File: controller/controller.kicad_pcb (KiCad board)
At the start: 4 copper layers, 30 x 60 mm, 74 parts, among them SW1 SW_SPDT, SW2 SW_SPST

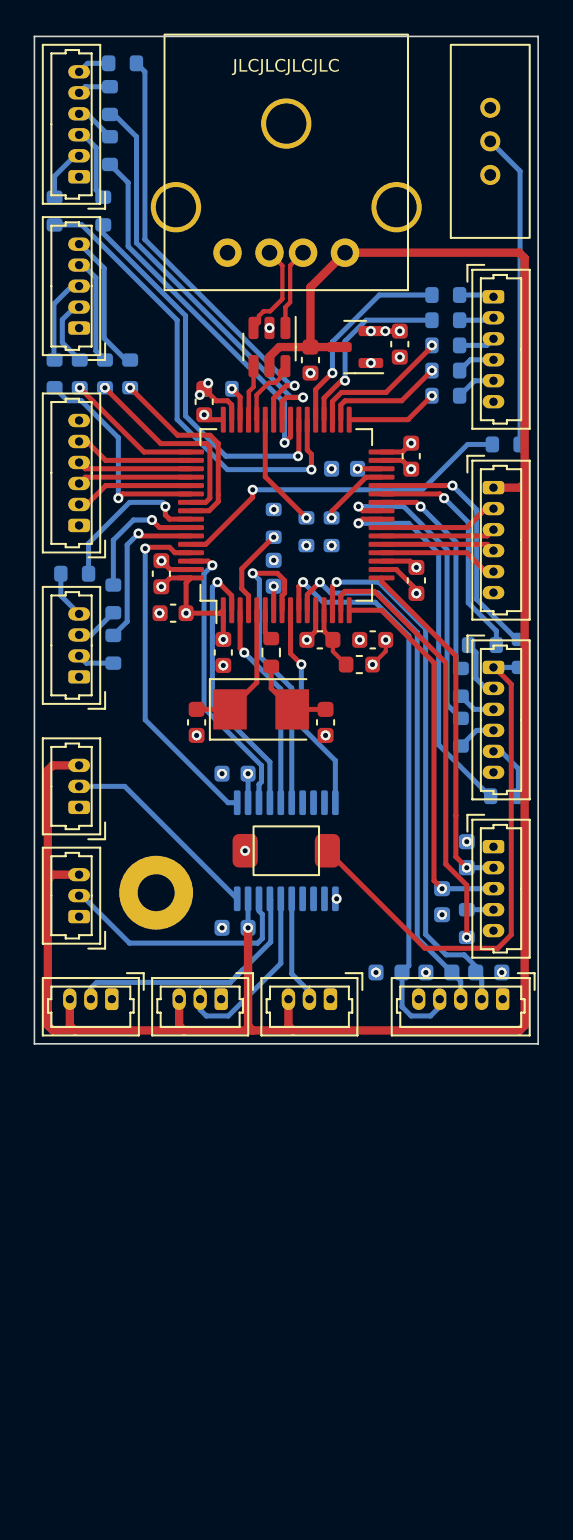
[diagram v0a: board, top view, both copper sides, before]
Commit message: update controller and host boards
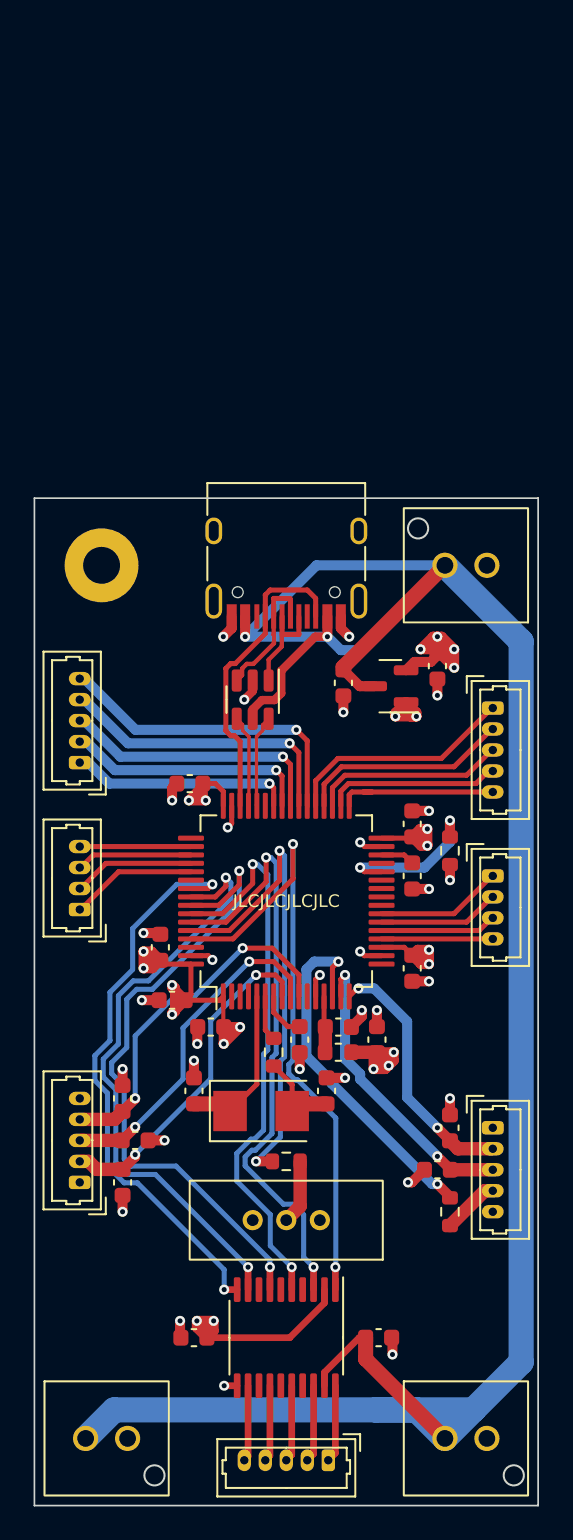
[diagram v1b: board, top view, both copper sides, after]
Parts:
- removed ESD1: USBLC6-2SC6, Package_TO_SOT_SMD:SOT-23-6
- removed H10, H11, H12, H13, H14: Conn_01x03, Connector_Molex:Molex_PicoBlade_53047-0310_1x03_P1.25mm_Vertical
- removed H2, H4, H5, H6: Conn_01x06, Connector_Molex:Molex_PicoBlade_53047-0610_1x06_P1.25mm_Vertical
- removed H3, H8, H9: Conn_01x05, Connector_Molex:Molex_PicoBlade_53047-0510_1x05_P1.25mm_Vertical
- removed H7: Conn_01x04, Connector_Molex:Molex_PicoBlade_53047-0410_1x04_P1.25mm_Vertical
- removed LDO1: AP2127N-3.3, Package_TO_SOT_SMD:SOT-23
- removed MCU1: STM32F401RCT6, Package_QFP:LQFP-64_10x10mm_P0.5mm
- removed MNT1: MountingHole, MountingHole:MountingHole_2.2mm_M2_Pad
- removed R10, R11, R12, R13, R14, R15, R16, R17, R18, R19, R20, R21, R22, R23, R24, R25, R26, R27, R28, R29, R5, R6, R7, R8, R9: 10KR, Resistor_SMD:R_0603_1608Metric
- removed SW2: SW_SPST, Custom:ALPS_SKRKAEE020
- removed USB1: USB_A, Custom:JST_UBA-4R-D14T-4D
- removed VT1: TXS0108EPW, Package_SO:TSSOP-20_4.4x6.5mm_P0.65mm
- removed XTAL1: 8MHz, Crystal:Crystal_SMD_5032-2Pin_5.0x3.2mm
- added J1: Conn_01x02, klib:MOLEX_533750210-Mini-Lock-2Pin-Through-Hole, F.Cu at (135.7, 74.0)
- added J10: Conn_01x05, Connector_Molex:Molex_PicoBlade_53047-0510_1x05_P1.25mm_Vertical, F.Cu at (137.3, 107.5)
- added J11: Conn_01x02, klib:MOLEX_533750210-Mini-Lock-2Pin-Through-Hole, F.Cu at (135.7, 126.0)
- added J2: USB_C_Receptacle_USB2.0, Connector_USB:USB_C_Receptacle_HRO_TYPE-C-31-M-12, F.Cu at (125.0, 73.0)
- added J3: Conn_01x02, klib:MOLEX_533750210-Mini-Lock-2Pin-Through-Hole, F.Cu at (114.3, 126.0)
- added J4: Conn_01x05, Connector_Molex:Molex_PicoBlade_53047-0510_1x05_P1.25mm_Vertical, F.Cu at (127.5, 127.3)
- added J5: Conn_01x04, Connector_Molex:Molex_PicoBlade_53047-0410_1x04_P1.25mm_Vertical, F.Cu at (112.7, 94.5)
- added J6: Conn_01x04, Connector_Molex:Molex_PicoBlade_53047-0410_1x04_P1.25mm_Vertical, F.Cu at (137.3, 92.5)
- added J7: Conn_01x05, Connector_Molex:Molex_PicoBlade_53047-0510_1x05_P1.25mm_Vertical, F.Cu at (112.7, 85.8)
- added J8: Conn_01x05, Connector_Molex:Molex_PicoBlade_53047-0510_1x05_P1.25mm_Vertical, F.Cu at (137.3, 82.5)
- added J9: Conn_01x05, Connector_Molex:Molex_PicoBlade_53047-0510_1x05_P1.25mm_Vertical, F.Cu at (112.7, 110.8)
- added U1: AP2127N-3.3, Package_TO_SOT_SMD:SOT-23, F.Cu at (131.2, 81.2)
- added U2: STM32F401RCT6, Package_QFP:LQFP-64_10x10mm_P0.5mm, F.Cu at (125.0, 94.0)
- added U3: USBLC6-2SC6, Package_TO_SOT_SMD:SOT-23-6, F.Cu at (123.0, 82.0)
- added U4: TXS0108EPW, Package_SO:TSSOP-20_4.4x6.5mm_P0.65mm, F.Cu at (125.0, 120.0)
- added Y1: 8M, Crystal:Crystal_SMD_5032-2Pin_5.0x3.2mm, F.Cu at (123.5, 106.5)
- C1, C2, C3, C9: value 10uF -> 10u
- C10, C4, C5, C6, C7, C8: value 100nF -> 100n
- C11: value 4.7uF -> 20p; moved to F.Cu
- C12: value 100nF -> 20p; moved to F.Cu
- C13: value 20pF -> 4.7u
- C14: value 20pF -> 100n
- C15, C16, C17, C18, C19, C20, C21: value 100nF -> 100n; moved to F.Cu
- H1: value Conn_01x06 -> MountingHole; footprint Connector_Molex:Molex_PicoBlade_53047-0610_1x06_P1.25mm_Vertical -> MountingHole:MountingHole_2.2mm_M2_Pad
- R1: value 0R -> 0
- R2, R3, R4: value 10KR -> 10K; moved to F.Cu
- SW1: footprint Custom:ALPS_SSSS912000 -> klib:ALPS_SSSS912000
- moved SW1 65.4 mm to (125.0, 113.0), turned to 180 degrees
- moved R4 53.4 mm to (134.8, 112.5)
- moved R2 44.7 mm to (125.0, 109.5), turned to 180 degrees
- moved C11 38.1 mm to (119.5, 105.3), turned to 90 degrees
- moved C15 33.0 mm to (119.5, 120.0), turned to 180 degrees
- moved C12 31.0 mm to (127.4, 105.3), turned to 90 degrees
- moved C16 26.2 mm to (130.5, 120.0), turned to 0 degrees
- moved C20 24.7 mm to (134.8, 107.5), turned to 90 degrees
- moved C9 23.8 mm to (130.4, 102.2), turned to 90 degrees
- moved R1 23.8 mm to (124.2, 103.0), turned to -90 degrees
- moved H1 23.8 mm to (114.0, 74.0), turned to 0 degrees
- moved FB1 23.1 mm to (128.1, 103.0)
- moved C5 23.1 mm to (132.5, 98.0)
- moved C10 23.1 mm to (128.1, 101.5), turned to 0 degrees
- moved C17 23.1 mm to (115.2, 105.8), turned to 90 degrees
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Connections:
- net +3.3VA renamed VREF
- C1 pad 1: VBUS -> 5V
- C11 pad 1: VCAP -> HSE_IN
- C12 pad 1: GND -> Net-(C12-Pad1)
- C12 pad 2: NRST -> GND
- C13 pad 1: HSE_IN -> VCAP
- C14 pad 1: Net-(C14-Pad1) -> NRST
- C15 pad 1: ST_X -> 3V3
- C16 pad 1: ST_Y -> 5V
- C2 pad 1: +3V3 -> 3V3
- C20 pad 1: GND -> ST_X
- C20 pad 2: +3V3 -> GND
- C21 pad 1: GND -> ST_Y
- C21 pad 2: VBUS -> GND
- C3 pad 1: +3V3 -> 3V3
- C4 pad 1: +3V3 -> 3V3
- C5 pad 1: +3V3 -> 3V3
- C6 pad 1: +3V3 -> 3V3
- C7 pad 1: +3V3 -> 3V3
- C8 pad 1: +3V3 -> 3V3
- C9 pad 1: +3V3 -> 3V3
- FB1 pad 1: +3V3 -> 3V3
- H1 pad 1: VBUS -> (no net)
- R1 pad 1: Net-(C14-Pad1) -> HSE_OUT
- R1 pad 2: HSE_OUT -> Net-(C12-Pad1)
- R2 pad 1: BOOT0 -> Net-(R2-Pad1)
- R2 pad 2: Net-(R2-Pad2) -> BOOT0
- R3 pad 1: BOOT1/KR1 -> BOOT1
- R3 pad 2: KR1 -> GND
- R4 pad 1: KT1 -> ST_P_IN
- R4 pad 2: KT1_IN -> ST_P
- SW1 pad 2: Net-(R2-Pad2) -> Net-(R2-Pad1)
- SW1 pad 3: +3V3 -> 3V3
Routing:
- net 5V: track 0.00 -> 145.5 mm, vias 0 -> 2
- net VBUS: track 131.6 -> 0.00 mm, vias 1 -> 0
- net 3V3: track 0.00 -> 70.4 mm, vias 0 -> 21
- net KR1: track 31.7 -> 0.00 mm
- net KI5: track 27.9 -> 0.00 mm, vias 1 -> 0
- net GND: track 12.6 -> 38.7 mm, vias 29 -> 33
- net KI1: track 26.1 -> 0.00 mm, vias 1 -> 0
- net LED4: track 12.5 -> 38.3 mm, vias 1 -> 2
- net KI2: track 24.8 -> 0.00 mm, vias 1 -> 0
- net KI4: track 23.3 -> 0.00 mm, vias 1 -> 0
- net KR5: track 22.8 -> 0.00 mm, vias 1 -> 0
- net KI3: track 22.4 -> 0.00 mm, vias 1 -> 0
- net LED_OE: track 12.6 -> 34.1 mm, vias 1 -> 2
- net COL1: track 0.00 -> 19.0 mm, vias 0 -> 1
- net +3V3: track 18.9 -> 0.00 mm, vias 12 -> 0
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- added copper zone on In2.Cu, net 3V3
- removed copper zone on In2.Cu, net +3V3
